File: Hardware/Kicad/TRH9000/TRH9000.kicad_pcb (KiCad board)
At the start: 4 copper layers, 100.1 x 73.4 mm, 63 parts, among them J1 RGB, Q1 BC817, U1 74HC138, U2 74HC32, U3 V9990, U4 KM428C256, U5 KM428C256, U6 LMH1980, X1 14.31818MHz, Y1 21.47727Mhz

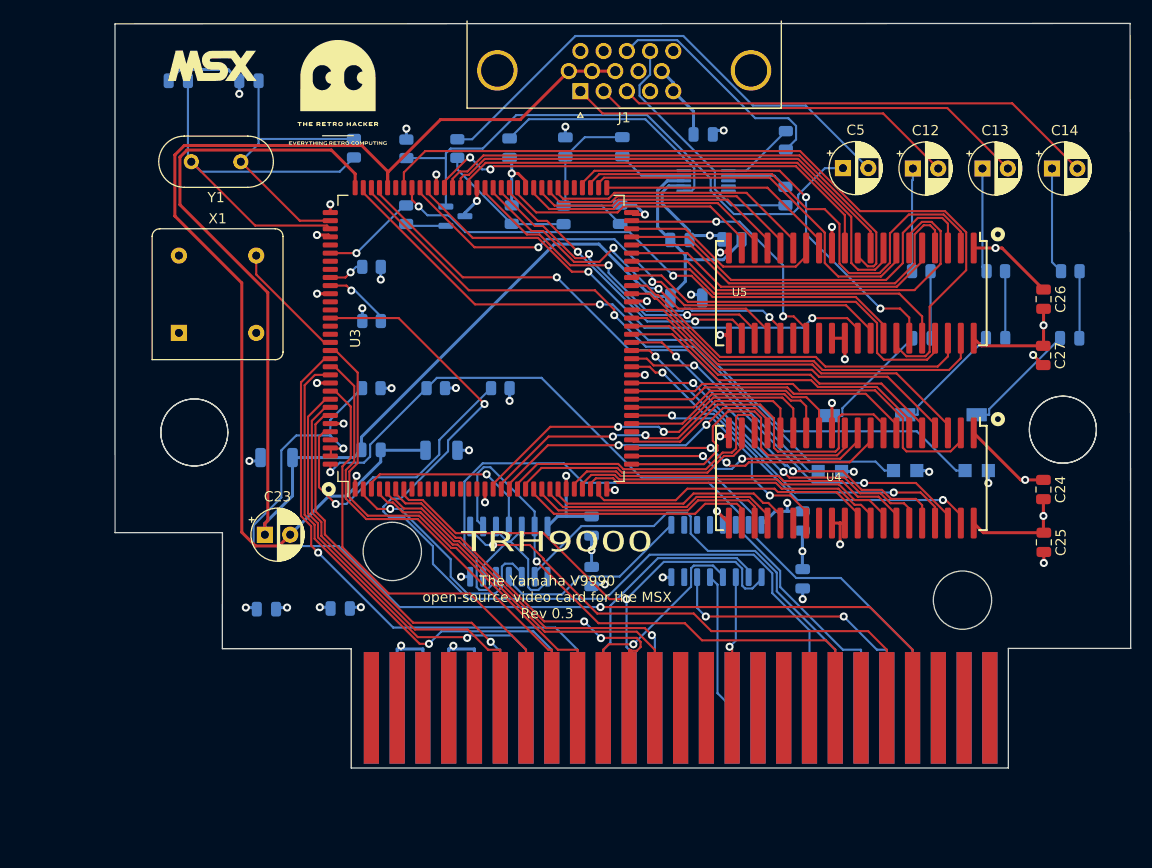
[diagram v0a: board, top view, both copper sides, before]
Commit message: Multiple changes.
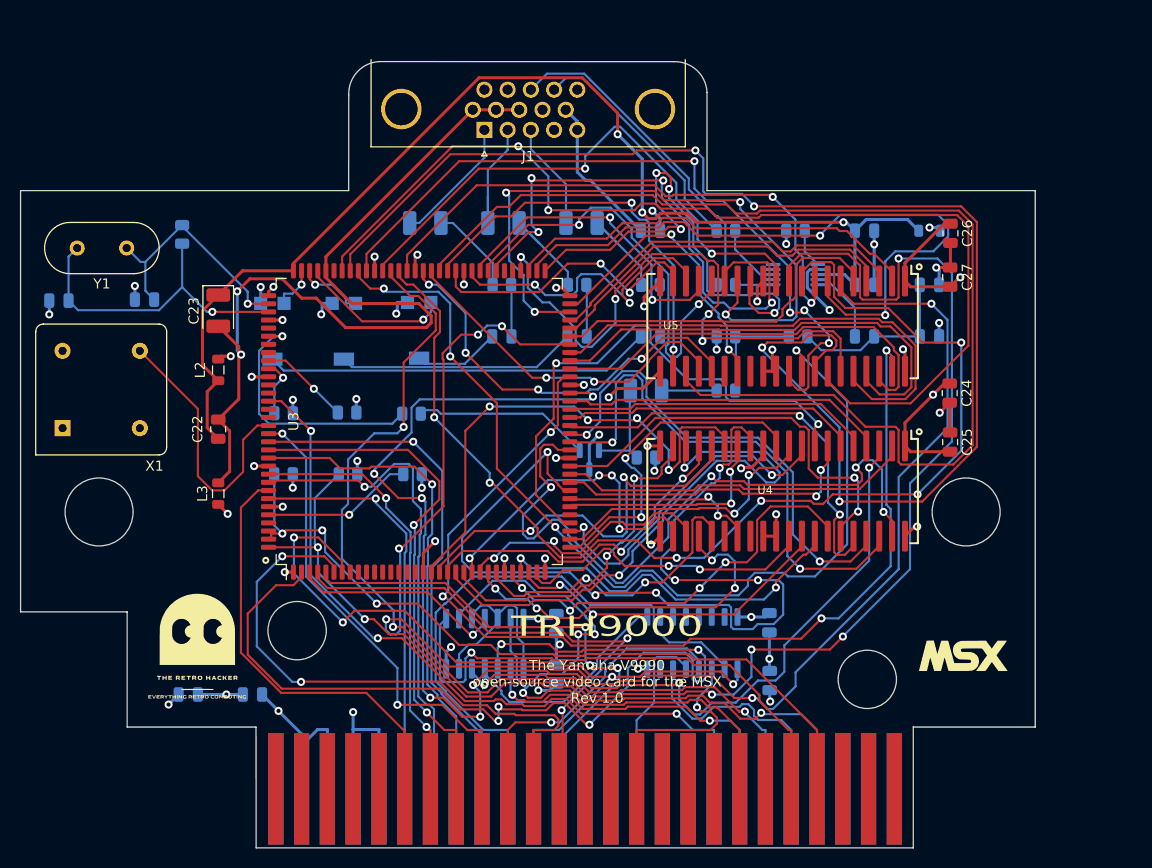
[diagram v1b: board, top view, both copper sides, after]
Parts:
- added REF**: OSHW-Logo2_9.8x8mm_SilkScreen, Symbol:OSHW-Logo2_9.8x8mm_SilkScreen, B.Cu at (182.4, 94.2)
- C11, C17: value 0.1µF -> 0.1uF
- C12, C13, C14: footprint Capacitor_THT:CP_Radial_D5.0mm_P2.50mm -> Capacitor_Tantalum_SMD:CP_EIA-3528-15_AVX-H; moved to B.Cu
- C15: value 10µF -> 10uF
- C18, C20: value 1 µF -> 1uF
- C2: value 1 µF -> 10uF
- C22: moved to F.Cu
- C23: footprint Capacitor_THT:CP_Radial_D5.0mm_P2.50mm -> Capacitor_Tantalum_SMD:CP_EIA-3528-15_AVX-H
- C5: value 220uF -> 220uF 6.3V; footprint Capacitor_THT:CP_Radial_D5.0mm_P2.50mm -> Capacitor_Tantalum_SMD:CP_EIA-3528-15_AVX-H; moved to B.Cu
- L1: value 4.7µH -> 4.7uH; footprint Inductor_SMD:L_1206_3216Metric -> Inductor_SMD:L_0805_2012Metric
- L2, L3: footprint Inductor_SMD:L_1206_3216Metric -> Inductor_SMD:L_0805_2012Metric; moved to F.Cu
- R12: value 10k -> 10K; footprint Capacitor_SMD:C_0805_2012Metric -> Resistor_SMD:R_0805_2012Metric
- moved MSX1 94.1 mm to (194.3, 114.6)
- moved RV3 70.3 mm to (126.2, 82.5), turned to 180 degrees
- moved RV2 56.4 mm to (133.3, 82.5), turned to 180 degrees
- moved TRH1 56.3 mm to (118.9, 113.5)
- moved C12 48.4 mm to (141.3, 71.9), turned to 180 degrees
- moved C13 47.5 mm to (149.0, 71.9), turned to 180 degrees
- moved C14 46.7 mm to (156.7, 71.9), turned to 180 degrees
- moved RV1 42.0 mm to (140.7, 82.5), turned to 180 degrees
- moved C6 41.4 mm to (148.9, 83.1)
- moved R17 41.4 mm to (163.5, 78.0)
- moved R15 41.4 mm to (148.9, 78.0)
- moved C8 41.3 mm to (163.5, 83.1)
- moved R16 41.3 mm to (156.3, 78.0)
- moved C7 41.2 mm to (156.3, 83.1)
- moved C10 40.5 mm to (191.0, 83.1), turned to 0 degrees
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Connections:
- BUS1 pad 12: /~{MERQ} -> unconnected-(BUS1-Pad12)
- C10 pad 1: Net-(C10-Pad1) -> Net-(C11-Pad1)
- C11 pad 1: /VIDEO/SYNCIN -> Net-(C11-Pad1)
- C11 pad 2: Net-(C10-Pad1) -> /VIDEO/SYNCIN
- C15 pad 1: GND -> GND1
- C15 pad 2: GND1 -> GND
- C16 pad 1: +5VA -> GND
- C16 pad 2: GND -> +5VA
- C9 pad 1: Net-(C10-Pad1) -> Net-(C11-Pad1)
- R11 pad 1: Net-(C10-Pad1) -> Net-(C11-Pad1)
- R12 pad 1: GND -> Net-(R12-Pad1)
- R12 pad 2: Net-(R12-Pad2) -> GND
- U6 pad 1: Net-(R12-Pad2) -> Net-(R12-Pad1)
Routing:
- net /VDP/V1D2: track 53.0 -> 163.8 mm, vias 0 -> 6
- net /VDP/V1S3: track 41.3 -> 147.2 mm, vias 0 -> 6
- net /VDP/V0S0: track 36.7 -> 126.1 mm, vias 0 -> 8
- net /VDP/V1D6: track 54.1 -> 141.0 mm, vias 2 -> 4
- net /VDP/V1A2: track 32.5 -> 114.4 mm, vias 2 -> 0
- net /VDP/~{V0_WE}: track 22.2 -> 91.6 mm, vias 0 -> 6
- net /VDP/~{VDPW}: track 24.4 -> 93.7 mm, vias 1 -> 5
- net /VDP/V1D1: track 46.7 -> 114.2 mm, vias 0 -> 6
- net /VDP/B: track 71.1 -> 4.41 mm
- net /VDP/V1S7: track 38.0 -> 100.3 mm, vias 0 -> 4
- net /VDP/G: track 63.6 -> 6.62 mm
- net Net-(C5-Pad1): track 57.2 -> 9.95 mm
- net /VDP/~{V1_RAS}: track 20.0 -> 64.7 mm, vias 0 -> 4
- net Net-(C5-Pad2): track 50.1 -> 5.42 mm
- net /VDP/V1D5: track 52.3 -> 96.2 mm, vias 2 -> 4
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- added copper zone on In2.Cu, net +5V
- added copper zone on In1.Cu, net GND
- removed copper zone on In1.Cu, net +5V
- removed copper zone on In2.Cu, net GND
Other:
- board size 100.1 x 73.4 mm -> 100 x 77.5 mm
- board text added: "The Yamaha V9990 open-source video card for the MSX Rev 1.0"
- board text removed: "The Yamaha V9990 open-source video card for the MSX Rev 0.3"
